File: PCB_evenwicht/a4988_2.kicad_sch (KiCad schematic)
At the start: 12 parts, among them IC1 A4988SETTR-T, J4 Conn_01x04_Pin

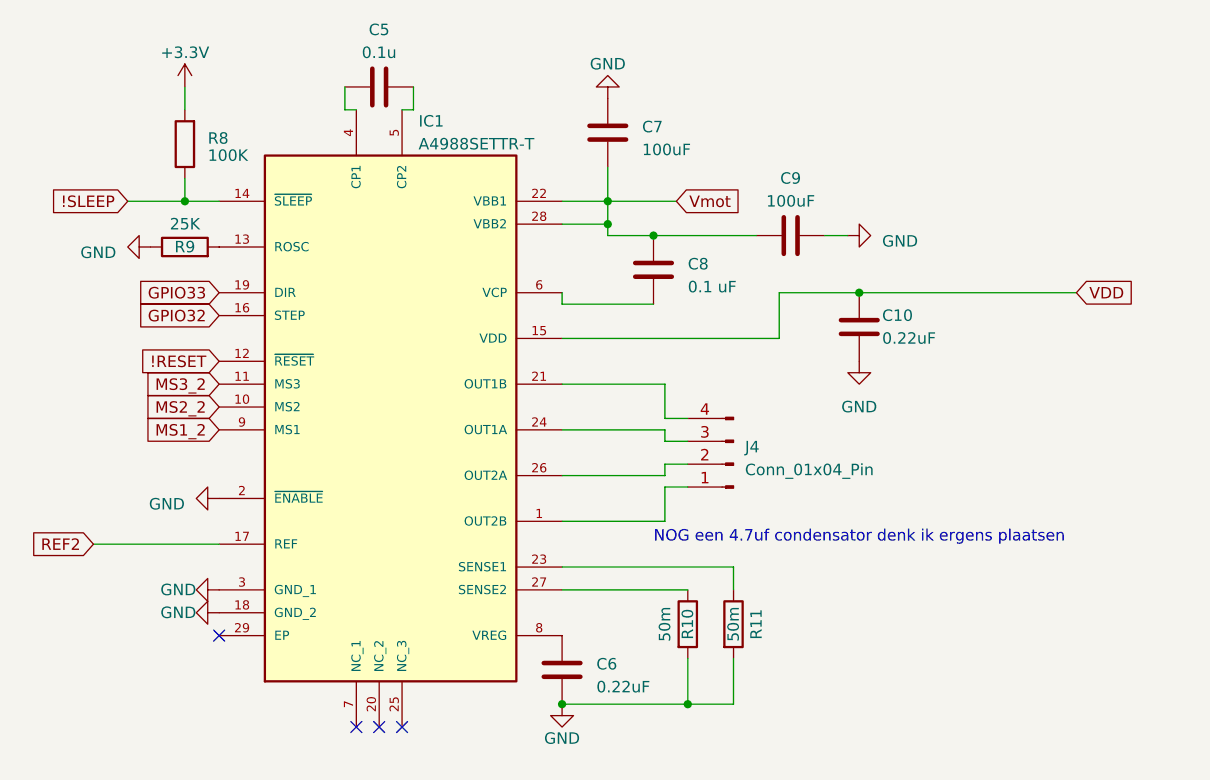
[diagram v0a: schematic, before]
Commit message: update pcb-design
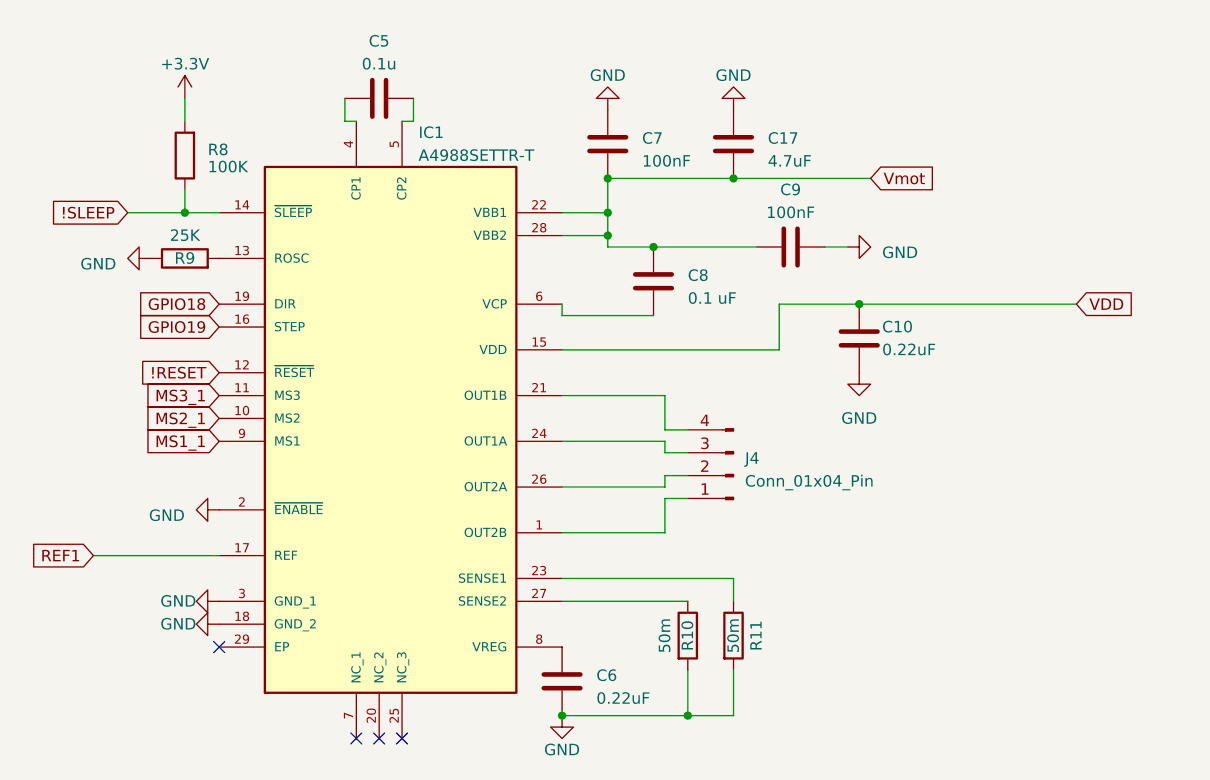
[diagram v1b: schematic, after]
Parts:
- added C17: 4.7uF, symbol Device:C
- C7, C9: value 100uF -> 100nF
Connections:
- net GND: now also C17.1
- net Vmot: now also C17.2
- net GPIO32 renamed GPIO19
- net GPIO33 renamed GPIO18
- net MS1_2 renamed MS1_1
- net MS2_2 renamed MS2_1
- net MS3_2 renamed MS3_1
- net REF2 renamed REF1
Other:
- note removed: "NOG een 4.7uf condensator denk ik ergens plaatsen"

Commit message: update pcb
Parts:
- C10, C17, C5, C6, C7, C8, C9: footprint (none) -> Capacitor_SMD:C_0603_1608Metric_Pad1.08x0.95mm_HandSolder
- R10, R11, R8, R9: footprint (none) -> Resistor_SMD:R_0805_2012Metric_Pad1.20x1.40mm_HandSolder
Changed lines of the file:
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@@
       (effects (font (size 1.27 1.27)))
     )
-    (property "Footprint" "" (at 54.61 55.118 90)
+    (property "Footprint" "Resistor_SMD:R_0805_2012Metric_Pad1.20x1.40mm_HandSolder" (at 54.61 55.118 90)
       (effects (font (size 1.27 1.27)) hide)
     )
@@
       (effects (font (size 1.27 1.27)))
     )
-    (property "Footprint" "" (at 113.792 95.25 90)
+    (property "Footprint" "Resistor_SMD:R_0805_2012Metric_Pad1.20x1.40mm_HandSolder" (at 113.792 95.25 90)
       (effects (font (size 1.27 1.27)) hide)
     )
@@
       (effects (font (size 1.27 1.27)))
     )
-    (property "Footprint" "" (at 108.712 95.25 90)
+    (property "Footprint" "Resistor_SMD:R_0805_2012Metric_Pad1.20x1.40mm_HandSolder" (at 108.712 95.25 90)
       (effects (font (size 1.27 1.27)) hide)
     )
@@
       (effects (font (size 1.27 1.27)) (justify right))
     )
-    (property "Footprint" "" (at 56.388 41.91 90)
+    (property "Footprint" "Resistor_SMD:R_0805_2012Metric_Pad1.20x1.40mm_HandSolder" (at 56.388 41.91 90)
       (effects (font (size 1.27 1.27)) hide)
     )
@@
       (effects (font (size 1.27 1.27)) (justify left))
     )
-    (property "Footprint" "" (at 97.4852 104.14 0)
+    (property "Footprint" "Capacitor_SMD:C_0603_1608Metric_Pad1.08x0.95mm_HandSolder" (at 97.4852 104.14 0)
       (effects (font (size 1.27 1.27)) hide)
     )
@@
       (effects (font (size 1.27 1.27)) (justify left))
     )
-    (property "Footprint" "" (at 116.5352 44.45 0)
+    (property "Footprint" "Capacitor_SMD:C_0603_1608Metric_Pad1.08x0.95mm_HandSolder" (at 116.5352 44.45 0)
       (effects (font (size 1.27 1.27)) hide)
     )
@@
       (effects (font (size 1.27 1.27)) (justify left))
     )
-    (property "Footprint" "" (at 102.5652 44.45 0)
+    (property "Footprint" "Capacitor_SMD:C_0603_1608Metric_Pad1.08x0.95mm_HandSolder" (at 102.5652 44.45 0)
       (effects (font (size 1.27 1.27)) hide)
     )
@@
       (effects (font (size 1.27 1.27)))
     )
-    (property "Footprint" "" (at 125.73 51.1048 0)
+    (property "Footprint" "Capacitor_SMD:C_0603_1608Metric_Pad1.08x0.95mm_HandSolder" (at 125.73 51.1048 0)
       (effects (font (size 1.27 1.27)) hide)
     )
@@
       (effects (font (size 1.27 1.27)) (justify left))
     )
-    (property "Footprint" "" (at 130.5052 66.04 0)
+    (property "Footprint" "Capacitor_SMD:C_0603_1608Metric_Pad1.08x0.95mm_HandSolder" (at 130.5052 66.04 0)
       (effects (font (size 1.27 1.27)) hide)
     )
@@
       (effects (font (size 1.27 1.27)) (justify left))
     )
-    (property "Footprint" "" (at 107.6452 59.69 0)
+    (property "Footprint" "Capacitor_SMD:C_0603_1608Metric_Pad1.08x0.95mm_HandSolder" (at 107.6452 59.69 0)
       (effects (font (size 1.27 1.27)) hide)
     )
@@
       (effects (font (size 1.27 1.27)))
     )
-    (property "Footprint" "" (at 72.39 36.5252 0)
-      (effects (font (size 1.27 1.27)) hide)
-    )
+    (property "Footprint" "Capacitor_SMD:C_0603_1608Metric_Pad1.08x0.95mm_HandSolder" (at 72.39 36.5252 0)
+      (effects (font (size 1.27 1.27)) hide)
+    )

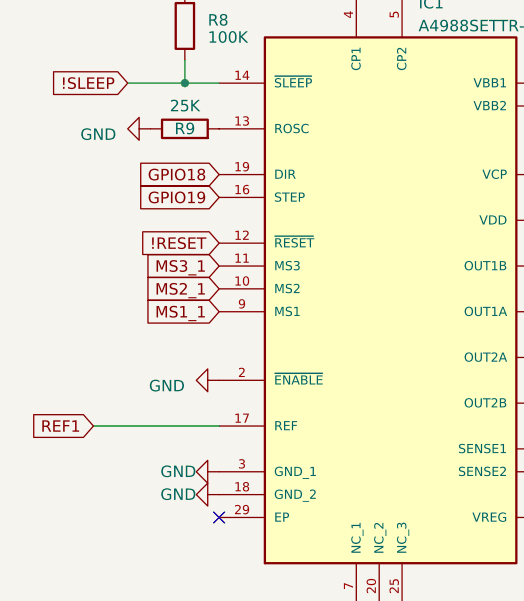
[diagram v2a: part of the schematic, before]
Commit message: klj
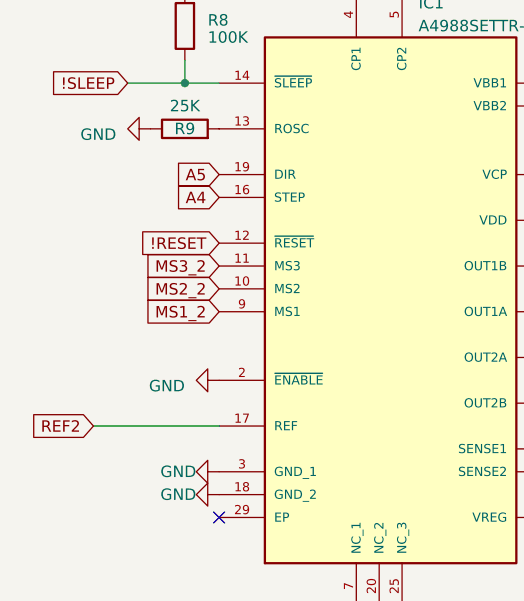
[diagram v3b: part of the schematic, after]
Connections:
- net GPIO18 renamed A5
- net GPIO19 renamed A4
- net MS1_1 renamed MS1_2
- net MS2_1 renamed MS2_2
- net MS3_1 renamed MS3_2
- net REF1 renamed REF2
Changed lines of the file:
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@@
     (stroke (width 0) (type default))
   )
-  (global_label "GPIO18" (shape input) (at 58.42 58.42 180) (fields_autoplaced)
+  (global_label "A5" (shape input) (at 58.42 58.42 180) (fields_autoplaced)
     (effects (font (size 1.27 1.27)) (justify right))
-    (property "Intersheetrefs" "${INTERSHEET_REFS}" (at 48.6199 58.42 0)
+    (property "Intersheetrefs" "${INTERSHEET_REFS}" (at 53.2161 58.42 0)
       (effects (font (size 1.27 1.27)) (justify right) hide)
     )
   )
-  (global_label "MS1_1" (shape input) (at 58.42 73.66 180) (fields_autoplaced)
+  (global_label "MS1_2" (shape input) (at 58.42 73.66 180) (fields_autoplaced)
     (effects (font (size 1.27 1.27)) (justify right))
     (property "Intersheetrefs" "${INTERSHEET_REFS}" (at 49.4667 73.66 0)
@@
     )
   )
-  (global_label "GPIO19" (shape input) (at 58.42 60.96 180) (fields_autoplaced)
+  (global_label "A4" (shape input) (at 58.42 60.96 180) (fields_autoplaced)
     (effects (font (size 1.27 1.27)) (justify right))
-    (property "Intersheetrefs" "${INTERSHEET_REFS}" (at 48.6199 60.96 0)
+    (property "Intersheetrefs" "${INTERSHEET_REFS}" (at 53.2161 60.96 0)
       (effects (font (size 1.27 1.27)) (justify right) hide)
     )
@@
     )
   )
-  (global_label "MS2_1" (shape input) (at 58.42 71.12 180) (fields_autoplaced)
+  (global_label "MS2_2" (shape input) (at 58.42 71.12 180) (fields_autoplaced)
     (effects (font (size 1.27 1.27)) (justify right))
     (property "Intersheetrefs" "${INTERSHEET_REFS}" (at 49.4667 71.12 0)
@@
     )
   )
-  (global_label "REF1" (shape input) (at 44.45 86.36 180) (fields_autoplaced)
+  (global_label "REF2" (shape input) (at 44.45 86.36 180) (fields_autoplaced)
     (effects (font (size 1.27 1.27)) (justify right))
     (property "Intersheetrefs" "${INTERSHEET_REFS}" (at 36.8271 86.36 0)
@@
     )
   )
-  (global_label "MS3_1" (shape input) (at 58.42 68.58 180) (fields_autoplaced)
+  (global_label "MS3_2" (shape input) (at 58.42 68.58 180) (fields_autoplaced)
     (effects (font (size 1.27 1.27)) (justify right))
     (property "Intersheetrefs" "${INTERSHEET_REFS}" (at 49.4667 68.58 0)
